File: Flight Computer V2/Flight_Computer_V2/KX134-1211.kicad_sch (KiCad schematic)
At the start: 8 parts, among them U4 KX134-1211

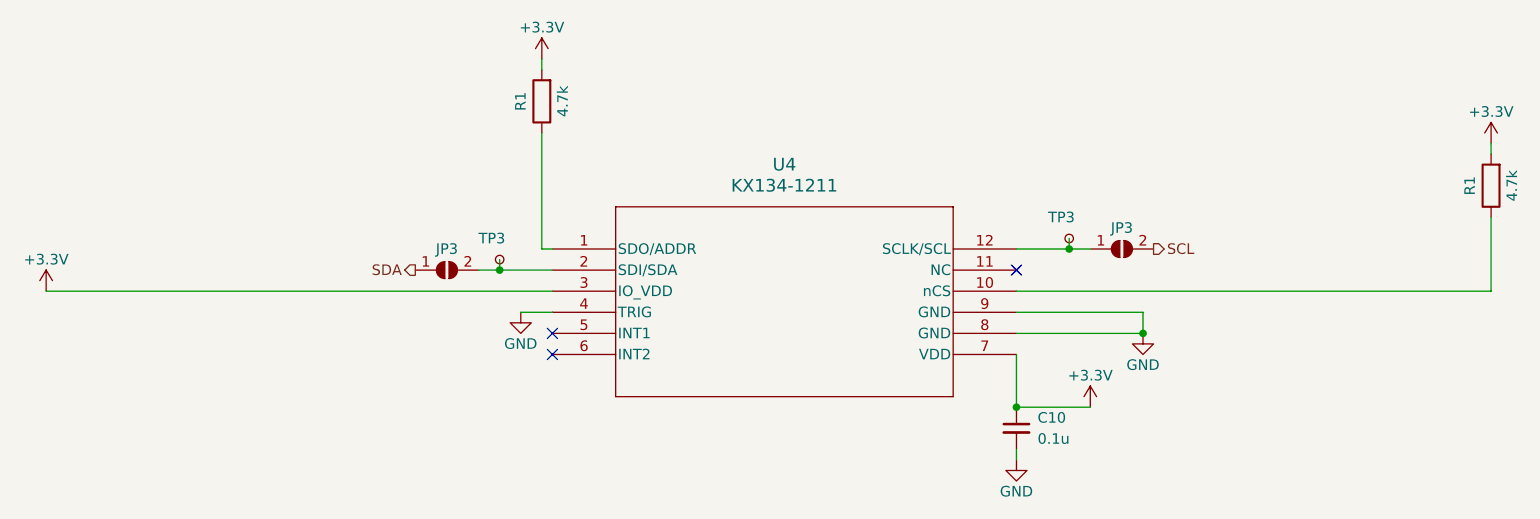
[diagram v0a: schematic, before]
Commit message: updated pcb
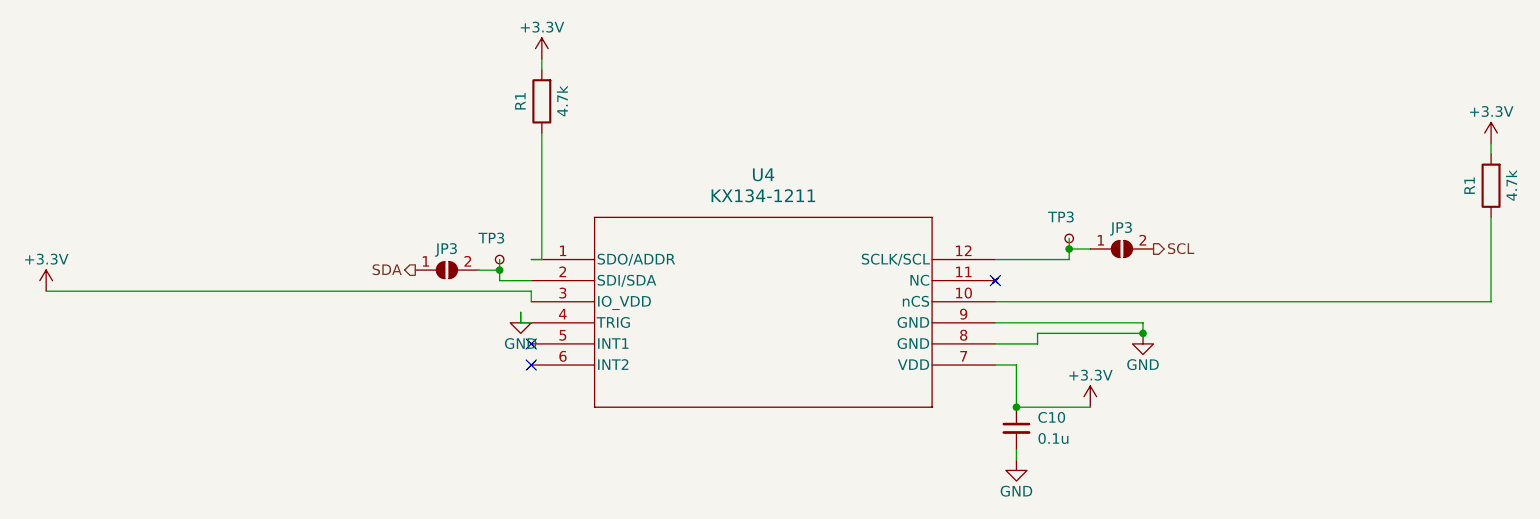
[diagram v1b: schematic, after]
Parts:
- C10: footprint (none) -> Capacitor_SMD:C_0402_1005Metric
- JP3: footprint (none) -> Jumper:SolderJumper-2_P1.3mm_Open_Pad1.0x1.5mm
- R1: footprint (none) -> Resistor_SMD:R_0402_1005Metric
- TP3: footprint (none) -> TestPoint:TestPoint_Pad_D1.0mm
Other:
- moved on the sheet: U4
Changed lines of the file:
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@@
   (junction (at 177.8 96.52) (diameter 0) (color 0 0 0 0)
   )
-  (no_connect (at 177.8 80.01))
-  (no_connect (at 121.92 90.17))
-  (no_connect (at 121.92 87.63))
-  (wire (pts (xy 60.96 82.55) (xy 121.92 82.55))
-    (stroke (width 0) (type default))
-  )
-  (wire (pts (xy 177.8 87.63) (xy 193.04 87.63))
-    (stroke (width 0) (type default))
-  )
-  (wire (pts (xy 120.65 77.47) (xy 121.92 77.47))
+  (no_connect (at 175.26 81.28))
+  (no_connect (at 119.38 91.44))
+  (no_connect (at 119.38 88.9))
+  (wire (pts (xy 184.15 78.74) (xy 184.15 77.47))
+    (stroke (width 0) (type default))
+  )
+  (wire (pts (xy 119.38 83.82) (xy 119.38 82.55))
+    (stroke (width 0) (type default))
+  )
+  (wire (pts (xy 175.26 91.44) (xy 177.8 91.44))
+    (stroke (width 0) (type default))
+  )
+  (wire (pts (xy 175.26 88.9) (xy 180.34 88.9))
+    (stroke (width 0) (type default))
+  )
+  (wire (pts (xy 120.65 78.74) (xy 119.38 78.74))
+    (stroke (width 0) (type default))
+  )
+  (wire (pts (xy 119.38 82.55) (xy 60.96 82.55))
     (stroke (width 0) (type default))
   )
@@
     (stroke (width 0) (type default))
   )
-  (wire (pts (xy 177.8 77.47) (xy 184.15 77.47))
+  (wire (pts (xy 175.26 78.74) (xy 184.15 78.74))
+    (stroke (width 0) (type default))
+  )
+  (wire (pts (xy 118.11 86.36) (xy 118.11 85.09))
     (stroke (width 0) (type default))
   )
@@
     (stroke (width 0) (type default))
   )
-  (wire (pts (xy 177.8 90.17) (xy 177.8 96.52))
-    (stroke (width 0) (type default))
-  )
   (wire (pts (xy 184.15 77.47) (xy 186.69 77.47))
     (stroke (width 0) (type default))
   )
-  (wire (pts (xy 193.04 87.63) (xy 193.04 85.09))
+  (wire (pts (xy 115.57 81.28) (xy 115.57 80.01))
+    (stroke (width 0) (type default))
+  )
+  (wire (pts (xy 177.8 91.44) (xy 177.8 96.52))
+    (stroke (width 0) (type default))
+  )
+  (wire (pts (xy 193.04 87.63) (xy 193.04 86.36))
     (stroke (width 0) (type default))
   )
@@
     (stroke (width 0) (type default))
   )
-  (wire (pts (xy 115.57 80.01) (xy 121.92 80.01))
-    (stroke (width 0) (type default))
-  )
-  (wire (pts (xy 193.04 85.09) (xy 177.8 85.09))
-    (stroke (width 0) (type default))
-  )
-  (wire (pts (xy 118.11 85.09) (xy 121.92 85.09))
+  (wire (pts (xy 115.57 81.28) (xy 119.38 81.28))
+    (stroke (width 0) (type default))
+  )
+  (wire (pts (xy 180.34 87.63) (xy 193.04 87.63))
+    (stroke (width 0) (type default))
+  )
+  (wire (pts (xy 193.04 86.36) (xy 175.26 86.36))
+    (stroke (width 0) (type default))
+  )
+  (wire (pts (xy 118.11 86.36) (xy 119.38 86.36))
     (stroke (width 0) (type default))
   )
@@
     (stroke (width 0) (type default))
   )
-  (wire (pts (xy 120.65 63.5) (xy 120.65 77.47))
-    (stroke (width 0) (type default))
-  )
-  (wire (pts (xy 177.8 82.55) (xy 234.95 82.55))
+  (wire (pts (xy 120.65 63.5) (xy 120.65 78.74))
+    (stroke (width 0) (type default))
+  )
+  (wire (pts (xy 180.34 88.9) (xy 180.34 87.63))
+    (stroke (width 0) (type default))
+  )
+  (wire (pts (xy 175.26 83.82) (xy 234.95 83.82))
     (stroke (width 0) (type default))
   )
@@
     (stroke (width 0) (type default))
   )
-  (wire (pts (xy 234.95 73.66) (xy 234.95 82.55))
+  (wire (pts (xy 234.95 73.66) (xy 234.95 83.82))
     (stroke (width 0) (type default))
   )
@@
       (effects (font (size 1.27 1.27)) (justify left) hide)
     )
-    (property "Footprint" "" (at 120.65 78.74 0)
+    (property "Footprint" "TestPoint:TestPoint_Pad_D1.0mm" (at 120.65 78.74 0)
       (effects (font (size 1.27 1.27)) hide)
     )
@@
       (effects (font (size 1.27 1.27)))
     )
-    (property "Footprint" "" (at 109.22 80.01 0)
+    (property "Footprint" "Jumper:SolderJumper-2_P1.3mm_Open_Pad1.0x1.5mm" (at 109.22 80.01 0)
       (effects (font (size 1.27 1.27)) hide)
     )
@@
       (effects (font (size 1.27 1.27)))
     )
-    (property "Footprint" "" (at 190.5 77.47 0)
+    (property "Footprint" "Jumper:SolderJumper-2_P1.3mm_Open_Pad1.0x1.5mm" (at 190.5 77.47 0)
       (effects (font (size 1.27 1.27)) hide)
     )
@@
       (effects (font (size 1.27 1.27)))
     )
-    (property "Footprint" "" (at 236.728 69.85 90)
+    (property "Footprint" "Resistor_SMD:R_0402_1005Metric" (at 236.728 69.85 90)
       (effects (font (size 1.27 1.27)) hide)
     )
@@
       (effects (font (size 1.27 1.27)))
     )
-    (property "Footprint" "" (at 122.428 59.69 90)
+    (property "Footprint" "Resistor_SMD:R_0402_1005Metric" (at 122.428 59.69 90)
       (effects (font (size 1.27 1.27)) hide)
     )
@@
       (effects (font (size 1.27 1.27)) (justify left) hide)
     )
-    (property "Footprint" "" (at 189.23 76.2 0)
+    (property "Footprint" "TestPoint:TestPoint_Pad_D1.0mm" (at 189.23 76.2 0)
       (effects (font (size 1.27 1.27)) hide)
     )
@@
     )
   )
-  (symbol (lib_id "KX134-1211:KX134-1211") (at 121.92 77.47 0) (unit 1)
+  (symbol (lib_id "KX134-1211:KX134-1211") (at 119.38 78.74 0) (unit 1)
     (in_bom yes) (on_board yes) (dnp no) (fields_autoplaced)
-    (property "Reference" "U4" (at 149.86 67.31 0)
+    (property "Reference" "U4" (at 147.32 68.58 0)
       (effects (font (size 1.524 1.524)))
     )
-    (property "Value" "KX134-1211" (at 149.86 69.85 0)
+    (property "Value" "KX134-1211" (at 147.32 71.12 0)
       (effects (font (size 1.524 1.524)))
     )
-    (property "Footprint" "LGA12_2X2X0P9_ROM" (at 121.92 77.47 0)
+    (property "Footprint" "LGA12_2X2X0P9_ROM" (at 119.38 78.74 0)
       (effects (font (size 1.27 1.27) italic) hide)
     )
-    (property "Datasheet" "KX134-1211" (at 121.92 77.47 0)
+    (property "Datasheet" "KX134-1211" (at 119.38 78.74 0)
       (effects (font (size 1.27 1.27) italic) hide)
     )
@@
       (effects (font (size 1.27 1.27)) (justify left))
     )
-    (property "Footprint" "" (at 177.8 99.06 0)
-      (effects (font (size 1.27 1.27)) hide)
-    )
+    (property "Footprint" "Capacitor_SMD:C_0402_1005Metric" (at 177.8 99.06 0)
+      (effects (font (size 1.27 1.27)) hide)
+    )
